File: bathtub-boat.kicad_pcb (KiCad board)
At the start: 2 copper layers, 55 x 38 mm, 11 parts, among them J1 I2C, J2 SPI, SW1 MODE, SW2 RESET, SW4 A, U1 esp-01m, U2 tp4056, U3 UA78M33_TO252, U4 DS18B20, U5 TTL

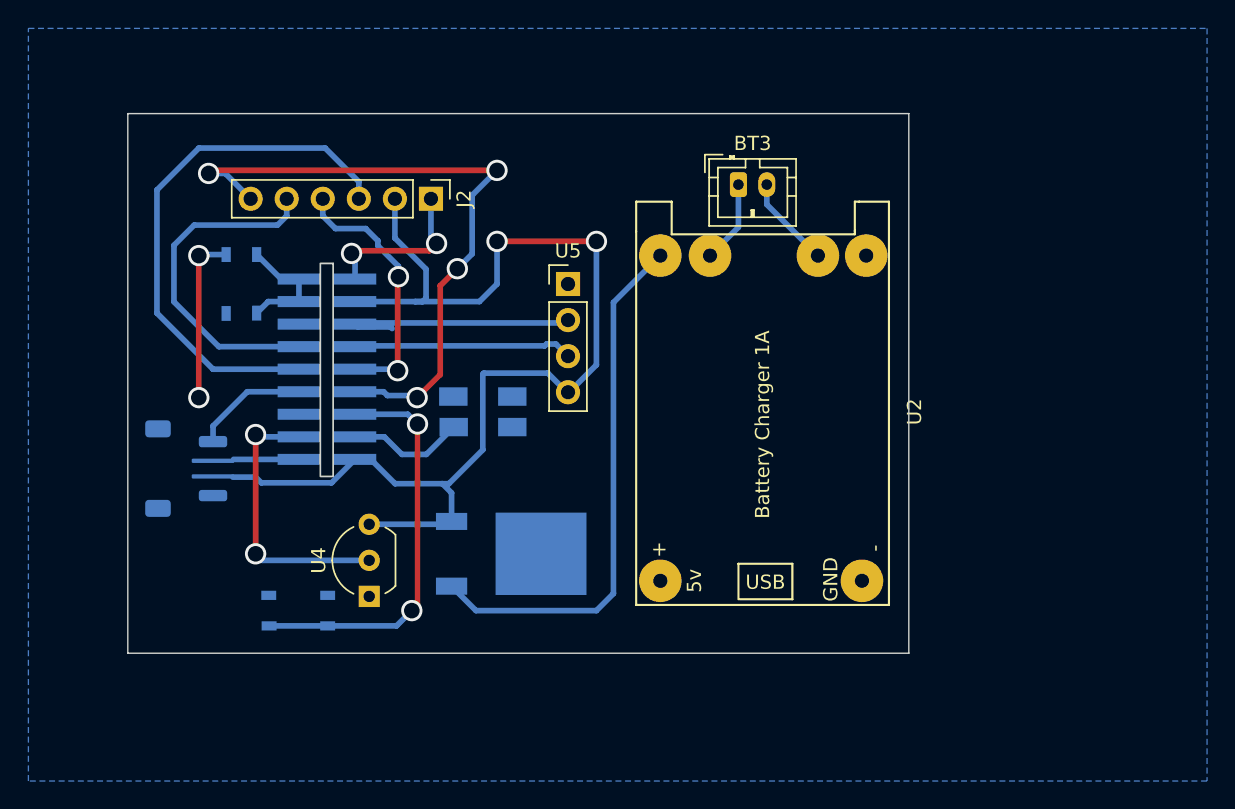
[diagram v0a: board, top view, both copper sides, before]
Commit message: Prepare for milling
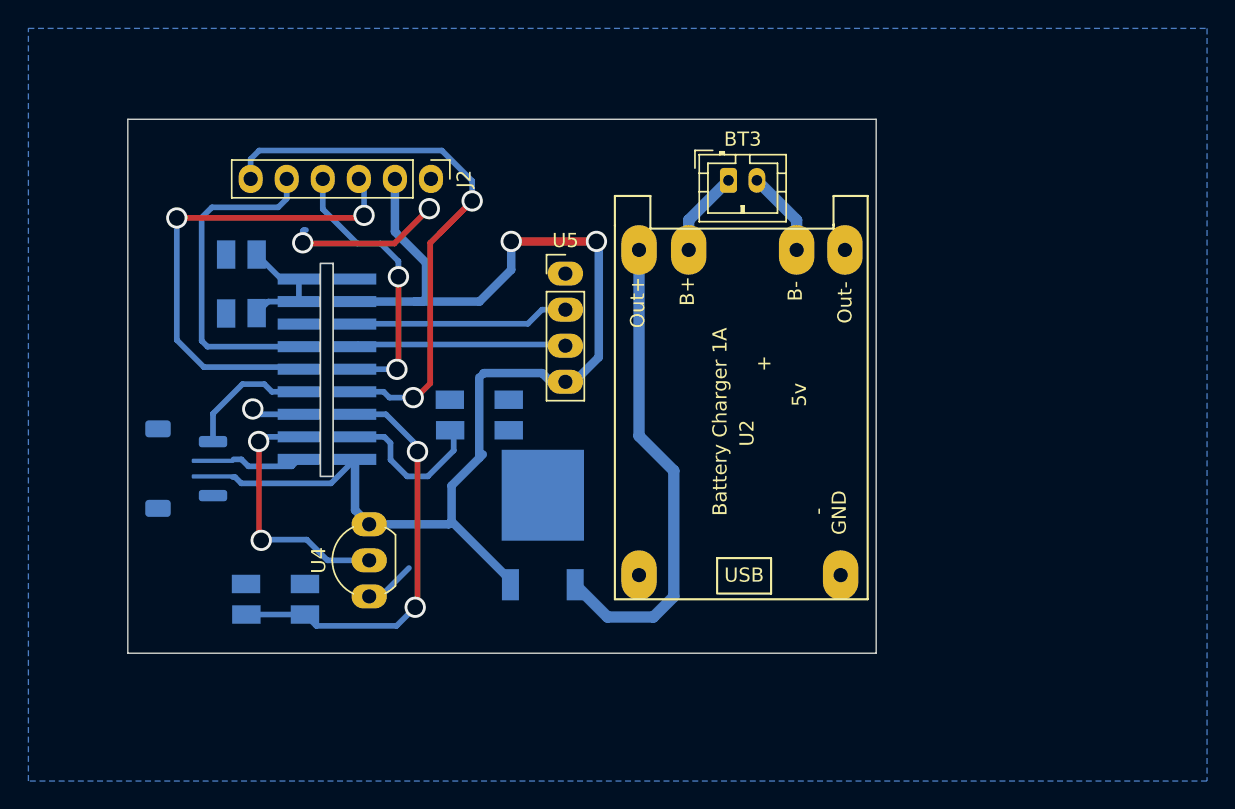
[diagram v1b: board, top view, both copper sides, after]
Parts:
- U2: value tp4056 -> TP4056
- moved U2 15.0 mm to (150.2, 54.5)
- moved U3 3.01 mm to (136.2, 62.0), turned to 90 degrees
- moved SW4 1.79 mm to (117.4, 67.2)
- moved J2 1.40 mm to (128.3, 37.6)
- moved BT3 0.76 mm to (149.3, 37.7)
- moved U5 0.76 mm to (137.8, 44.3)
- moved SW1 0.34 mm to (131.8, 54.2)
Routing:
- net GND: track 23.4 -> 14.7 mm, vias 4 -> 2
- net +3V3: track 81.6 -> 86.2 mm
- net SPI_CS: track 47.0 -> 42.7 mm, vias 4 -> 2
- net +5V: track 37.8 -> 33.9 mm
- net SPI_MISO: track 37.9 -> 34.4 mm, vias 0 -> 2
- net Neopixel: track 0.00 -> 3.41 mm, vias 0 -> 1
- net Net-(SW1-Pad2): track 8.26 -> 11.2 mm
- net TX: track 17.9 -> 15.4 mm
- net TEMP: track 19.7 -> 18.2 mm
- net BUTTON-A: track 28.5 -> 29.5 mm
- net I2C_SCL: track 8.25 -> 9.21 mm
- net SPI_MOSI: track 18.6 -> 19.6 mm
- net RX: track 15.5 -> 15.0 mm
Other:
- board size 55 x 38 mm -> 52.7 x 37.6 mm
